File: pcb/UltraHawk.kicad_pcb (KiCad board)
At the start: 2 copper layers, 50 x 87 mm, 80 parts, among them J1 USB_C_Receptacle_USB2.0_16P, J10 Screw_Terminal_01x02, J11 Conn_01x03_Pin, J12 Conn_01x03_Pin, J13 Conn_01x03_Pin, J14 Conn_01x03_Pin, J15 Conn_01x03_Pin, J2 Conn_01x04_Pin, J3 Conn_01x03_Pin, J4 Conn_01x04_Pin, J5 Conn_01x04_Pin, J6 Conn_01x06_Pin, J7 Screw_Terminal_01x02, J8 Screw_Terminal_01x02, J9 Screw_Terminal_01x02, SW1 TS-1088R-02026, U1 STM32H723VGTx, U2 AMS1117-3.3, U3 BMI270, U4 BMP581, U5 LIS3MDL, U6 TPS565208, U7 AO3400A, U8 AO3400A, U9 AO3400A, Y1 16MHZ

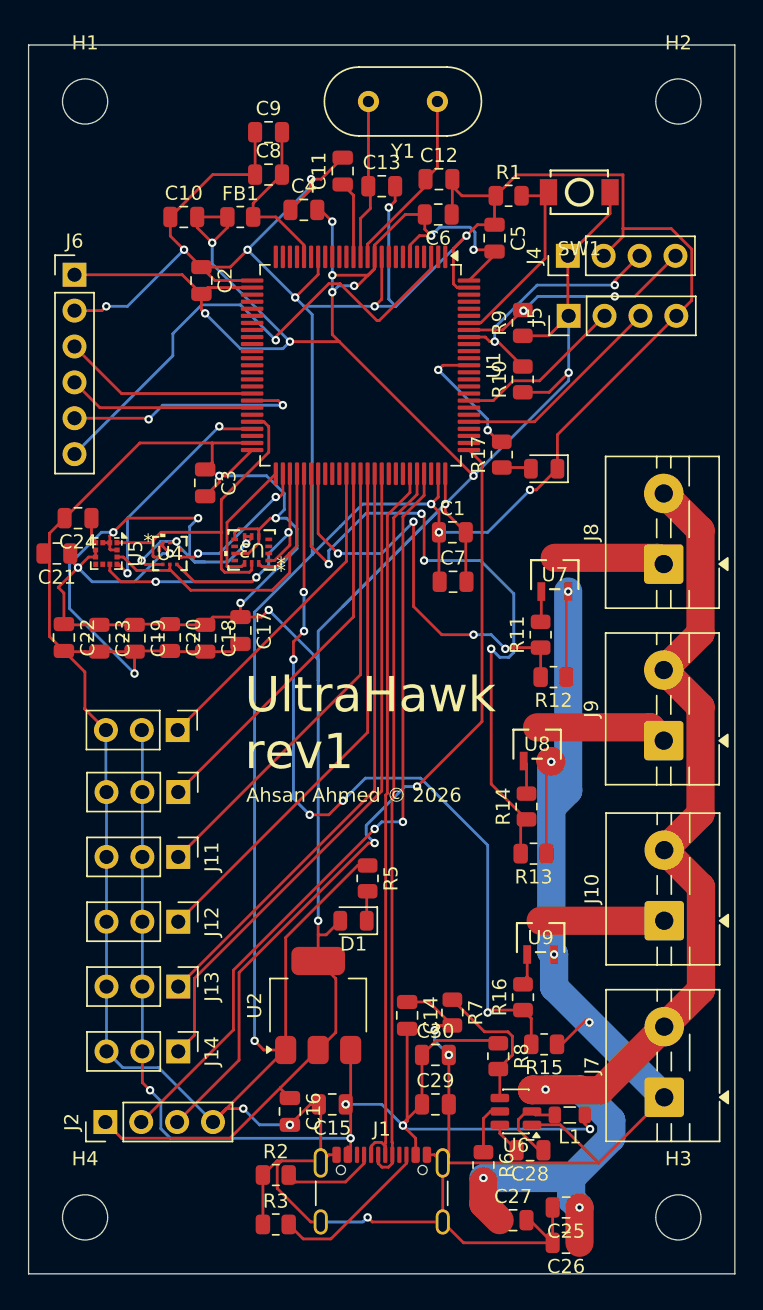
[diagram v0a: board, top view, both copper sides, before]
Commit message: DRC fixes
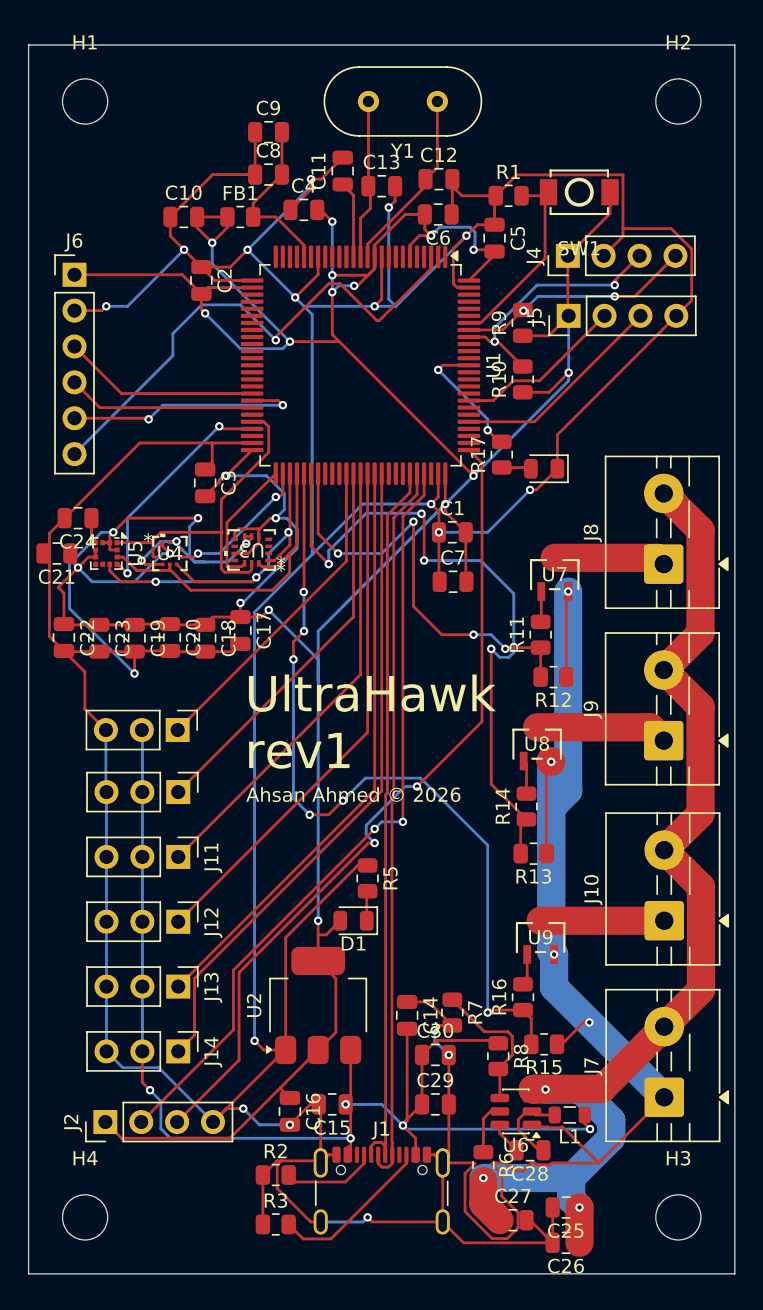
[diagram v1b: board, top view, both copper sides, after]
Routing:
- net GND: track 519.6 -> 532.9 mm
- net 3.3V: track 276.6 -> 275.8 mm
